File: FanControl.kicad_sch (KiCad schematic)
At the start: 22 parts, among them M1 Fan_3pin, Q4 Q_PMOS_DGS, Q5 Q_NMOS_DGS, U5 LM4040DBZ-3

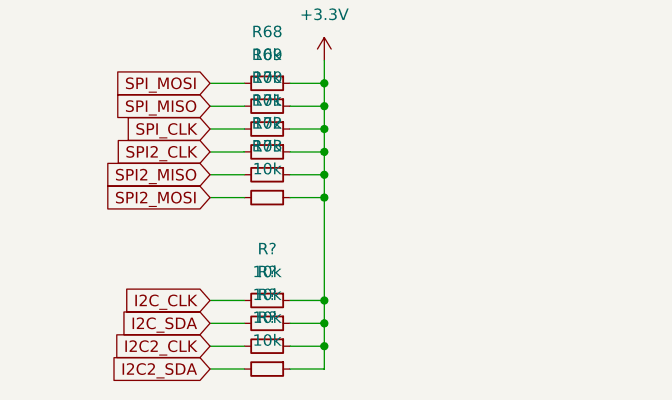
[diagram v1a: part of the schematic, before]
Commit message: j
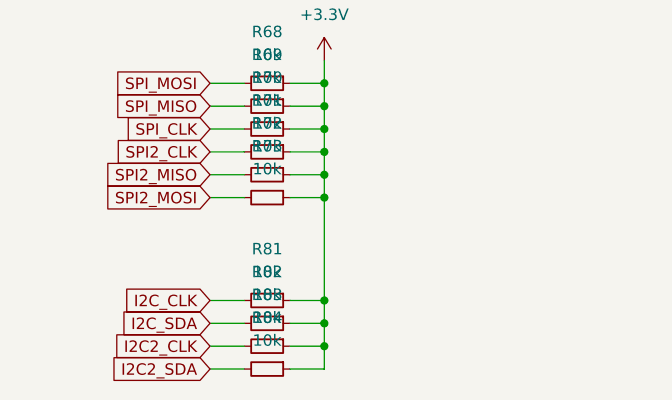
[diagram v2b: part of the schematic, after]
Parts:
- gave numbers to parts that had none: 4
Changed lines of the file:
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@@
   (symbol (lib_id "Device:R_Small") (at 38.735 157.48 270) (unit 1)
     (in_bom yes) (on_board yes) (fields_autoplaced)
-    (property "Reference" "R?" (id 0) (at 38.735 151.765 90))
+    (property "Reference" "R84" (id 0) (at 38.735 151.765 90))
     (property "Value" "10k" (id 1) (at 38.735 154.305 90))
     (property "Footprint" "Resistor_SMD:R_0603_1608Metric_Pad0.98x0.95mm_HandSolder" (id 2) (at 38.735 157.48 0)
@@
   (symbol (lib_id "Device:R_Small") (at 38.735 149.86 270) (unit 1)
     (in_bom yes) (on_board yes) (fields_autoplaced)
-    (property "Reference" "R?" (id 0) (at 38.735 144.145 90))
+    (property "Reference" "R81" (id 0) (at 38.735 144.145 90))
     (property "Value" "10k" (id 1) (at 38.735 146.685 90))
     (property "Footprint" "Resistor_SMD:R_0603_1608Metric_Pad0.98x0.95mm_HandSolder" (id 2) (at 38.735 149.86 0)
@@
   (symbol (lib_id "Device:R_Small") (at 38.735 154.94 270) (unit 1)
     (in_bom yes) (on_board yes) (fields_autoplaced)
-    (property "Reference" "R?" (id 0) (at 38.735 149.225 90))
+    (property "Reference" "R83" (id 0) (at 38.735 149.225 90))
     (property "Value" "10k" (id 1) (at 38.735 151.765 90))
     (property "Footprint" "Resistor_SMD:R_0603_1608Metric_Pad0.98x0.95mm_HandSolder" (id 2) (at 38.735 154.94 0)
@@
   (symbol (lib_id "Device:R_Small") (at 38.735 152.4 270) (unit 1)
     (in_bom yes) (on_board yes) (fields_autoplaced)
-    (property "Reference" "R?" (id 0) (at 38.735 146.685 90))
+    (property "Reference" "R82" (id 0) (at 38.735 146.685 90))
     (property "Value" "10k" (id 1) (at 38.735 149.225 90))
     (property "Footprint" "Resistor_SMD:R_0603_1608Metric_Pad0.98x0.95mm_HandSolder" (id 2) (at 38.735 152.4 0)
